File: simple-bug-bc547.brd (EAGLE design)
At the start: 25.4 x 20.3 mm, 13 parts, among them T1 BC547

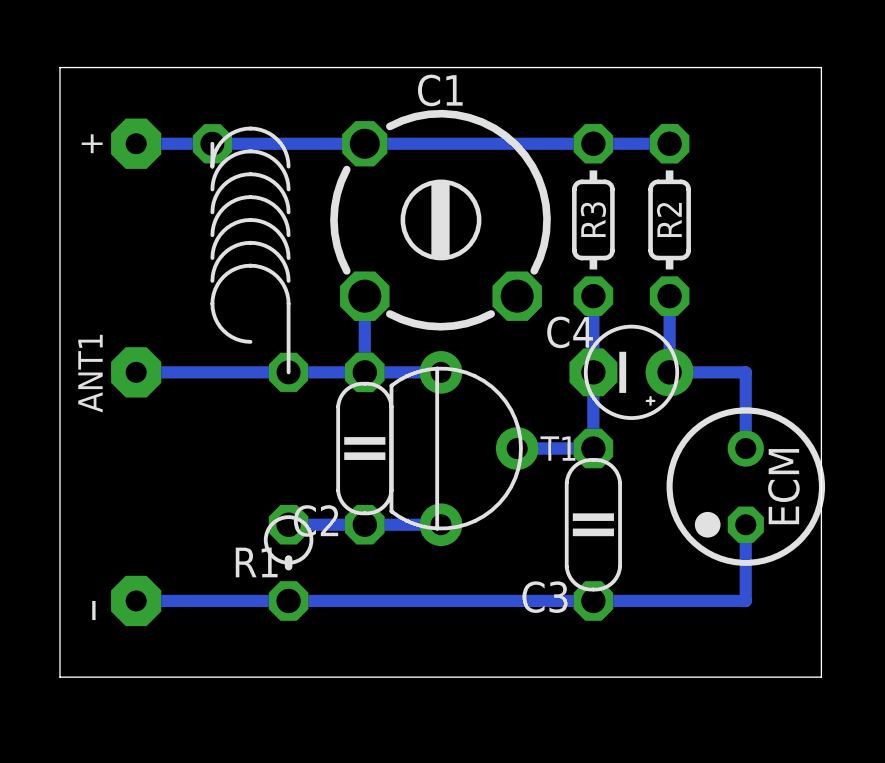
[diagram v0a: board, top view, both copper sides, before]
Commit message: ...
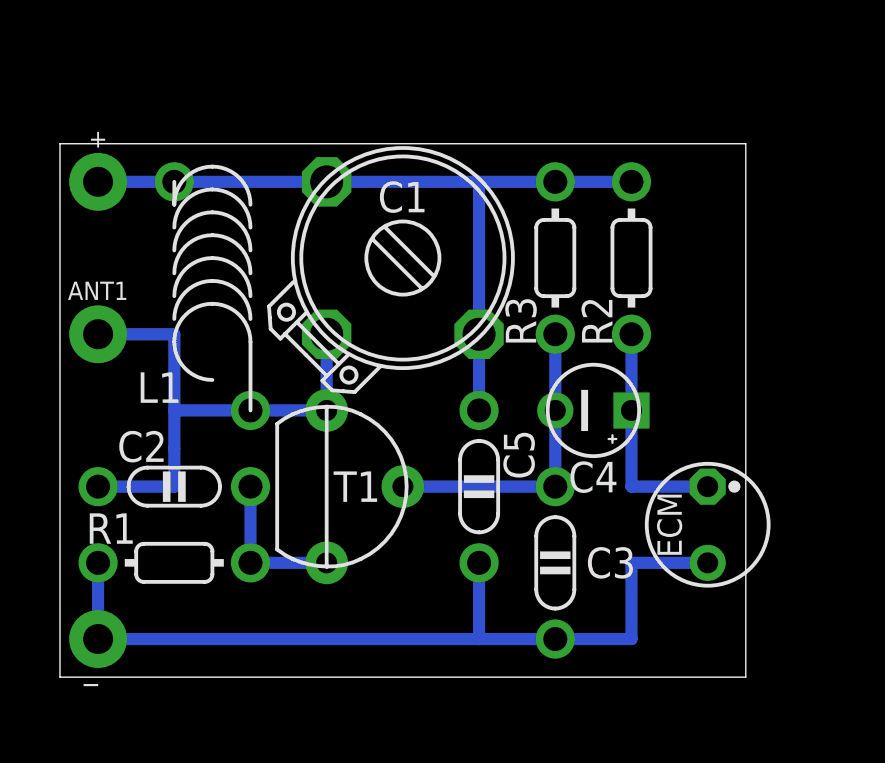
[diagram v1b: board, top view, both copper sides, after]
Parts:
- added C5: 22nF, c:C050-020X036
- C1: value C-TR-PH20127-45-2P23 -> 1.6-15pF; device cap-trim:TRIM808-45 -> cap-trim:TRIM-2222-808
- C3: device c:C050-020X036 -> c:C050-020X036/V
- C4: value (none) -> 1uF
- ECM: value ECM-5 -> ECM-4; device ECM:ECM-5 -> ECM:ECM-4
- L1: device r:L-04/7 -> r:L-04/7V
- R1: device r:0202V -> r:0202/5
- R2: value 22k -> 4.7k
- moved C2 6.48 mm to (3.81, 6.35)
- moved T1 4.02 mm to (8.89, 6.35), turned to 0 degrees
- moved R1 3.81 mm to (3.81, 3.81)
- moved ̶̶ 1.80 mm to (1.27, 1.27), turned to 90 degrees
- moved + 1.80 mm to (1.27, 16.5), turned to 270 degrees
- moved ANT1 1.80 mm to (1.27, 11.4), turned to 270 degrees
- moved C3 1.80 mm to (16.5, 3.81), turned to 180 degrees
- moved C1 1.80 mm to (11.4, 14.0)
- moved C4 1.80 mm to (17.8, 8.89), turned to 270 degrees
- moved ECM 1.80 mm to (21.6, 5.08), turned to 0 degrees
- moved R2 1.80 mm to (19.1, 14.0), turned to 90 degrees
- moved R3 1.80 mm to (16.5, 14.0), turned to 90 degrees
- moved L1 1.27 mm to (5.08, 14.0)
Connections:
- net +UB: now also +.1, C1.1, C5.1; no longer +.P
- net GND: now also C5.2, ECM.2, ̶̶.1; no longer ECM.1, ̶̶.P
- net N$1: now also ANT1.1; no longer ANT1.P
- net N$6: now also ECM.1; no longer ECM.2
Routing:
- net +UB: track 17.8 -> 25.4 mm
- net N$1: track 12.7 -> 17.8 mm
- net GND: track 22.9 -> 27.9 mm
- net N$5: track 7.62 -> 10.2 mm
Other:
- board size 25.4 x 20.3 mm -> 22.9 x 17.8 mm
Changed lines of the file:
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@@
 <layer number="25" name="tNames" color="7" fill="1" visible="yes" active="yes"/>
 <layer number="26" name="bNames" color="7" fill="1" visible="yes" active="yes"/>
-<layer number="27" name="tValues" color="7" fill="1" visible="no" active="yes"/>
-<layer number="28" name="bValues" color="7" fill="1" visible="no" active="yes"/>
+<layer number="27" name="tValues" color="7" fill="1" visible="yes" active="yes"/>
+<layer number="28" name="bValues" color="7" fill="1" visible="yes" active="yes"/>
 <layer number="29" name="tStop" color="7" fill="3" visible="no" active="yes"/>
 <layer number="30" name="bStop" color="7" fill="6" visible="no" active="yes"/>
@@
 <board>
 <plain>
-<wire x1="0" y1="0" x2="25.38" y2="0" width="0" layer="20"/>
-<wire x1="25.38" y1="0" x2="25.38" y2="20.32" width="0" layer="20"/>
-<wire x1="25.38" y1="20.32" x2="0" y2="20.32" width="0" layer="20"/>
-<wire x1="0" y1="20.32" x2="0" y2="0" width="0" layer="20"/>
+<wire x1="0" y1="0" x2="22.86" y2="0" width="0" layer="20"/>
+<wire x1="22.86" y1="0" x2="22.86" y2="17.78" width="0" layer="20"/>
+<wire x1="22.86" y1="17.78" x2="0" y2="17.78" width="0" layer="20"/>
+<wire x1="0" y1="17.78" x2="0" y2="0" width="0" layer="20"/>
 </plain>
 <attributes>
@@
 </autorouter>
 <elements>
-<element name="C2" library="c" package="C050-020X036" value="4.7pF" x="10.16" y="7.62"/>
-<element name="C3" library="c" package="C050-020X036" value="1nF" x="17.78" y="5.08"/>
-<element name="L1" library="r" package="L-04/7" value="1uH" x="6.35" y="13.97"/>
-<element name="R2" library="r" package="0202/5" value="22k" x="20.32" y="15.24"/>
-<element name="R3" library="r" package="0202/5" value="47k" x="17.78" y="15.24"/>
-<element name="T1" library="t" package="TO92-CBE-A" value="BC547" x="12.7" y="7.62" rot="R180"/>
-<element name="ECM" library="ECM" package="ECM-5" value="ECM-5" x="22.86" y="6.35" rot="R180"/>
-<element name="C1" library="cap-trim" package="TRIM808-45" value="C-TR-PH20127-45-2P23" x="12.7" y="15.24"/>
-<element name="R1" library="r" package="0202V" value="" x="7.62" y="3.81"/>
-<element name="C4" library="c" package="E2,5-3" value="" x="19.05" y="10.16"/>
-<element name="+" library="pad" package="SPAD" value="SPAD" x="2.54" y="17.78" rot="R180"/>
-<element name="̶̶" library="pad" package="SPAD" value="SPAD" x="2.54" y="2.54" rot="R180"/>
-<element name="ANT1" library="pad" package="SPAD" value="ANT" x="2.54" y="10.16" rot="R180"/>
+<element name="C2" library="c" package="C050-020X036" value="4.7pF" x="3.81" y="6.35"/>
+<element name="C3" library="c" package="C050-020X036/V" value="1nF" x="16.51" y="3.81" rot="R180"/>
+<element name="L1" library="r" package="L-04/7V" value="1uH" x="5.08" y="13.97"/>
+<element name="R2" library="r" package="0202/5" value="4.7k" x="19.05" y="13.97" rot="R90"/>
+<element name="R3" library="r" package="0202/5" value="47k" x="16.51" y="13.97" rot="R90"/>
+<element name="T1" library="t" package="TO92-CBE-A" value="BC547" x="8.89" y="6.35"/>
+<element name="ECM" library="ECM" package="ECM-4" value="ECM-4" x="21.59" y="5.08"/>
+<element name="C1" library="cap-trim" package="TRIM-2222-808" value="1.6-15pF" x="11.43" y="13.97"/>
+<element name="R1" library="r" package="0202/5" value="" x="3.81" y="3.81"/>
+<element name="C4" library="c" package="E2,5-3" value="1uF" x="17.78" y="8.89" rot="R270"/>
+<element name="+" library="pad" package="SPAD" value="SPAD" x="1.27" y="16.51" rot="R270"/>
+<element name="̶̶" library="pad" package="SPAD" value="SPAD" x="1.27" y="1.27" rot="R90"/>
+<element name="ANT1" library="pad" package="SPAD" value="ANT" x="1.27" y="11.43" rot="R270"/>
+<element name="C5" library="c" package="C050-020X036" value="22nF" x="13.97" y="6.35" rot="R270"/>
 </elements>
 <signals>
@@
 <contactref element="T1" pad="C"/>
 <contactref element="C2" pad="1"/>
+<contactref element="ANT1" pad="1"/>
+<wire x1="6.35" y1="8.89" x2="3.81" y2="8.89" width="0.4064" layer="16"/>
+<wire x1="3.81" y1="8.89" x2="3.81" y2="7.62" width="0.4064" layer="16"/>
+<wire x1="1.27" y1="6.35" x2="3.81" y2="6.35" width="0.4064" layer="16"/>
+<wire x1="3.81" y1="6.35" x2="3.81" y2="7.62" width="0.4064" layer="16"/>
+<wire x1="3.81" y1="8.89" x2="3.81" y2="11.43" width="0.4064" layer="16"/>
+<wire x1="3.81" y1="11.43" x2="1.27" y2="11.43" width="0.4064" layer="16"/>
 <contactref element="C1" pad="2"/>
-<contactref element="ANT1" pad="P"/>
-<wire x1="10.16" y1="10.16" x2="7.62" y2="10.16" width="0.4064" layer="16"/>
-<wire x1="10.16" y1="10.16" x2="12.7" y2="10.16" width="0.4064" layer="16"/>
-<wire x1="10.16" y1="10.16" x2="10.16" y2="12.7" width="0.4064" layer="16"/>
-<wire x1="7.62" y1="10.16" x2="2.54" y2="10.16" width="0.4064" layer="16"/>
+<wire x1="8.89" y1="8.89" x2="8.89" y2="11.43" width="0.4064" layer="16"/>
+<wire x1="8.89" y1="8.89" x2="6.35" y2="8.89" width="0.4064" layer="16"/>
 </signal>
 <signal name="N$3">
@@
 <contactref element="T1" pad="E"/>
 <contactref element="R1" pad="2"/>
-<wire x1="10.16" y1="5.08" x2="7.62" y2="5.08" width="0.4064" layer="16"/>
-<wire x1="10.16" y1="5.08" x2="12.7" y2="5.08" width="0.4064" layer="16"/>
+<wire x1="6.35" y1="6.35" x2="6.35" y2="3.81" width="0.4064" layer="16"/>
+<wire x1="6.35" y1="3.81" x2="8.89" y2="3.81" width="0.4064" layer="16"/>
 </signal>
 <signal name="N$5">
@@
 <contactref element="T1" pad="B"/>
 <contactref element="C4" pad="-"/>
-<wire x1="15.24" y1="7.62" x2="17.78" y2="7.62" width="0.4064" layer="16"/>
-<wire x1="17.78" y1="10.16" x2="17.78" y2="12.7" width="0.4064" layer="16"/>
-<wire x1="17.78" y1="10.16" x2="17.78" y2="7.62" width="0.4064" layer="16"/>
+<wire x1="16.51" y1="8.89" x2="16.51" y2="11.43" width="0.4064" layer="16"/>
+<wire x1="16.51" y1="8.89" x2="16.51" y2="6.35" width="0.4064" layer="16"/>
+<wire x1="11.43" y1="6.35" x2="16.51" y2="6.35" width="0.4064" layer="16"/>
 </signal>
 <signal name="N$6">
 <contactref element="R2" pad="1"/>
-<contactref element="ECM" pad="2"/>
 <contactref element="C4" pad="+"/>
-<wire x1="20.32" y1="10.16" x2="22.86" y2="10.16" width="0.4064" layer="16"/>
-<wire x1="22.86" y1="10.16" x2="22.86" y2="7.62" width="0.4064" layer="16"/>
-<wire x1="20.32" y1="10.16" x2="20.32" y2="12.7" width="0.4064" layer="16"/>
+<wire x1="19.05" y1="8.89" x2="19.05" y2="6.35" width="0.4064" layer="16"/>
+<wire x1="19.05" y1="8.89" x2="19.05" y2="11.43" width="0.4064" layer="16"/>
+<contactref element="ECM" pad="1"/>
+<wire x1="21.59" y1="6.35" x2="19.05" y2="6.35" width="0.4064" layer="16"/>
 </signal>
 <signal name="GND">
 <contactref element="C3" pad="2"/>
-<contactref element="ECM" pad="1"/>
 <contactref element="R1" pad="1"/>
-<contactref element="̶̶" pad="P"/>
-<wire x1="22.86" y1="2.54" x2="22.86" y2="5.08" width="0.4064" layer="16"/>
-<wire x1="17.78" y1="2.54" x2="22.86" y2="2.54" width="0.4064" layer="16"/>
-<wire x1="2.54" y1="2.54" x2="7.62" y2="2.54" width="0.4064" layer="16"/>
-<wire x1="7.62" y1="2.54" x2="17.78" y2="2.54" width="0.4064" layer="16"/>
+<contactref element="̶̶" pad="1"/>
+<wire x1="16.51" y1="1.27" x2="19.05" y2="1.27" width="0.4064" layer="16"/>
+<wire x1="19.05" y1="1.27" x2="19.05" y2="3.81" width="0.4064" layer="16"/>
+<wire x1="1.27" y1="3.81" x2="1.27" y2="1.27" width="0.4064" layer="16"/>
+<wire x1="1.27" y1="1.27" x2="13.97" y2="1.27" width="0.4064" layer="16"/>
+<contactref element="C5" pad="2"/>
+<wire x1="13.97" y1="1.27" x2="16.51" y2="1.27" width="0.4064" layer="16"/>
+<wire x1="13.97" y1="3.81" x2="13.97" y2="1.27" width="0.4064" layer="16"/>
+<contactref element="ECM" pad="2"/>
+<wire x1="19.05" y1="3.81" x2="21.59" y2="3.81" width="0.4064" layer="16"/>
 </signal>
 <signal name="+UB">
@@
 <contactref element="R3" pad="2"/>
 <contactref element="R2" pad="2"/>
+<contactref element="C1" pad="1"/>
+<contactref element="+" pad="1"/>
+<wire x1="19.05" y1="16.51" x2="16.51" y2="16.51" width="0.4064" layer="16"/>
+<wire x1="1.27" y1="16.51" x2="3.81" y2="16.51" width="0.4064" layer="16"/>
+<wire x1="3.81" y1="16.51" x2="8.89" y2="16.51" width="0.4064" layer="16"/>
+<wire x1="8.89" y1="16.51" x2="13.97" y2="16.51" width="0.4064" layer="16"/>
+<contactref element="C5" pad="1"/>
 <contactref element="C1" pad="3"/>
-<contactref element="+" pad="P"/>
-<wire x1="20.32" y1="17.78" x2="17.78" y2="17.78" width="0.4064" layer="16"/>
-<wire x1="2.54" y1="17.78" x2="5.08" y2="17.78" width="0.4064" layer="16"/>
-<wire x1="5.08" y1="17.78" x2="10.16" y2="17.78" width="0.4064" layer="16"/>
-<wire x1="10.16" y1="17.78" x2="17.78" y2="17.78" width="0.4064" layer="16"/>
+<wire x1="13.97" y1="16.51" x2="16.51" y2="16.51" width="0.4064" layer="16"/>
+<wire x1="13.97" y1="8.89" x2="13.97" y2="11.43" width="0.4064" layer="16"/>
+<wire x1="13.97" y1="11.43" x2="13.97" y2="16.51" width="0.4064" layer="16"/>
 </signal>
 </signals>
